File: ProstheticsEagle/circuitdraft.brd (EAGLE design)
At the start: 60 x 29.8 mm, 48 parts, among them IC1 BQ25887RGER, IC2 TPS54627DDAR, Q1 16 MHz

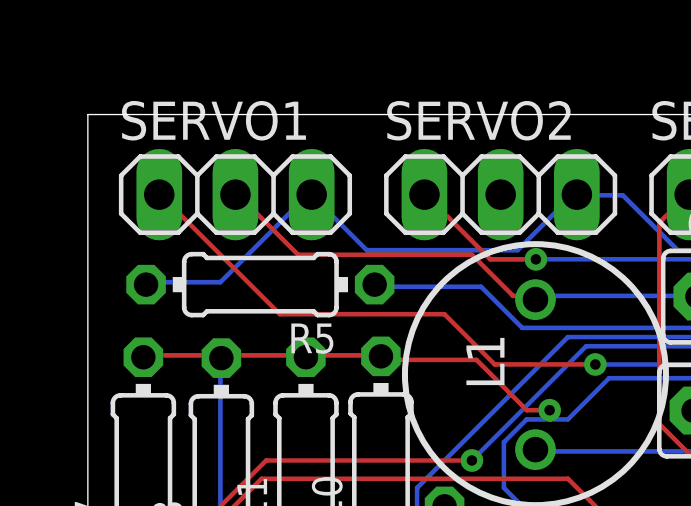
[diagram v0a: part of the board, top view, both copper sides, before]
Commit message: LED
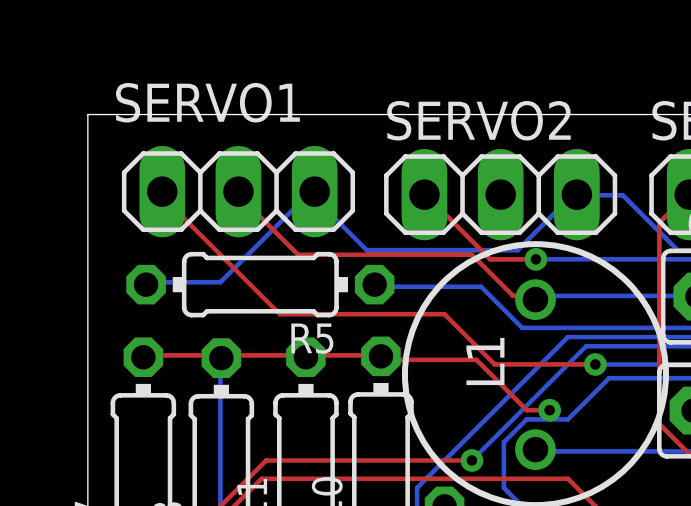
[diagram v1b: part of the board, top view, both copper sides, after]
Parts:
- moved SERVO1 0.14 mm to (5.02, 27.2)
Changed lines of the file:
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@@
 <drawing>
 <settings>
-<setting alwaysvectorfont="yes"/>
+<setting alwaysvectorfont="no"/>
 <setting verticaltext="up"/>
 </settings>
@@
 <attribute name="VALUE" x="35.0474" y="11.1456" size="0.9906" layer="27" ratio="10" rot="R270"/>
 </element>
-<element name="SERVO1" library="pinhead" library_urn="urn:adsk.eagle:library:325" package="1X03" package3d_urn="urn:adsk.eagle:package:22458/2" value="" x="4.92" y="27.15" smashed="yes">
-<attribute name="NAME" x="1.0338" y="28.9788" size="1.27" layer="25" ratio="10"/>
-<attribute name="POPULARITY" value="92" x="58.26" y="-18.57" size="1.778" layer="27" display="off"/>
-<attribute name="VALUE" x="1.11" y="23.975" size="1.27" layer="27"/>
+<element name="SERVO1" library="pinhead" library_urn="urn:adsk.eagle:library:325" package="1X03" package3d_urn="urn:adsk.eagle:package:22458/2" value="" x="5.02" y="27.25" smashed="yes">
+<attribute name="NAME" x="0.8338" y="29.5788" size="1.27" layer="25" ratio="10"/>
+<attribute name="POPULARITY" value="92" x="58.36" y="-18.47" size="1.778" layer="27" display="off"/>
+<attribute name="VALUE" x="1.21" y="24.075" size="1.27" layer="27"/>
 </element>
 <element name="SERVO2" library="pinhead" library_urn="urn:adsk.eagle:library:325" package="1X03" package3d_urn="urn:adsk.eagle:package:22458/2" value="" x="13.76" y="27.15" smashed="yes">
@@
 <wire x1="14.9352" y1="23.7744" x2="14.92" y2="23.65" width="0.1524" layer="16"/>
 <wire x1="20.2692" y1="23.7744" x2="20.32" y2="23.75" width="0.1524" layer="16"/>
-<wire x1="7.0104" y1="25.146" x2="5.0292" y2="27.1272" width="0.1524" layer="1"/>
+<wire x1="7.0104" y1="25.146" x2="5.049978125" y2="27.106421875" width="0.1524" layer="1"/>
 <wire x1="12.8016" y1="25.146" x2="7.0104" y2="25.146" width="0.1524" layer="1"/>
 <wire x1="14.1732" y1="23.7744" x2="12.8016" y2="25.146" width="0.1524" layer="1"/>
 <wire x1="14.7828" y1="23.7744" x2="14.1732" y2="23.7744" width="0.1524" layer="1"/>
-<wire x1="5.0292" y1="27.1272" x2="4.92" y2="27.15" width="0.1524" layer="1"/>
+<wire x1="5.049978125" y1="27.106421875" x2="5.02" y2="27.25" width="0.1524" layer="1"/>
 <wire x1="14.7828" y1="23.7744" x2="14.92" y2="23.65" width="0.1524" layer="1"/>
 <wire x1="22.5552" y1="25.908" x2="22.5552" y2="27.1272" width="0.1524" layer="1"/>
@@
 <wire x1="23.622" y1="10.8204" x2="23.56" y2="10.95" width="0.1524" layer="1"/>
 <wire x1="4.4196" y1="24.2316" x2="1.9812" y2="24.2316" width="0.1524" layer="16"/>
-<wire x1="7.3152" y1="27.1272" x2="4.4196" y2="24.2316" width="0.1524" layer="16"/>
+<wire x1="7.4152" y1="27.2272" x2="4.4196" y2="24.2316" width="0.1524" layer="16"/>
 <wire x1="1.9812" y1="24.2316" x2="1.94" y2="24.15" width="0.1524" layer="16"/>
-<wire x1="7.3152" y1="27.1272" x2="7.46" y2="27.15" width="0.1524" layer="16"/>
+<wire x1="7.4152" y1="27.2272" x2="7.56" y2="27.25" width="0.1524" layer="16"/>
 <wire x1="14.3256" y1="25.2984" x2="16.1544" y2="27.1272" width="0.1524" layer="16"/>
 <wire x1="9.2964" y1="25.2984" x2="14.3256" y2="25.2984" width="0.1524" layer="16"/>
-<wire x1="7.4676" y1="27.1272" x2="9.2964" y2="25.2984" width="0.1524" layer="16"/>
+<wire x1="7.6676" y1="26.9272" x2="9.2964" y2="25.2984" width="0.1524" layer="16"/>
 <wire x1="16.1544" y1="27.1272" x2="16.3" y2="27.15" width="0.1524" layer="16"/>
-<wire x1="7.4676" y1="27.1272" x2="7.46" y2="27.15" width="0.1524" layer="16"/>
+<wire x1="7.6676" y1="26.9272" x2="7.56" y2="27.25" width="0.1524" layer="16"/>
 <wire x1="25.146" y1="24.9936" x2="25.146" y2="27.1272" width="0.1524" layer="1"/>
 <wire x1="27.7368" y1="22.4028" x2="25.146" y2="24.9936" width="0.1524" layer="1"/>
@@
 <wire x1="11.8872" y1="23.1648" x2="13.5636" y2="21.4884" width="0.1524" layer="1"/>
 <wire x1="6.4008" y1="23.1648" x2="11.8872" y2="23.1648" width="0.1524" layer="1"/>
-<wire x1="2.4384" y1="27.1272" x2="6.4008" y2="23.1648" width="0.1524" layer="1"/>
+<wire x1="2.585290625" y1="26.980309375" x2="6.4008" y2="23.1648" width="0.1524" layer="1"/>
 <wire x1="51.6636" y1="22.86" x2="51.69" y2="22.79" width="0.1524" layer="1"/>
-<wire x1="2.4384" y1="27.1272" x2="2.38" y2="27.15" width="0.1524" layer="1"/>
+<wire x1="2.585290625" y1="26.980309375" x2="2.48" y2="27.25" width="0.1524" layer="1"/>
 <via x="46.9392" y="22.86" extent="1-16" drill="0.35"/>
 <via x="16.9164" y="21.4884" extent="1-16" drill="0.35"/>

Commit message: reste
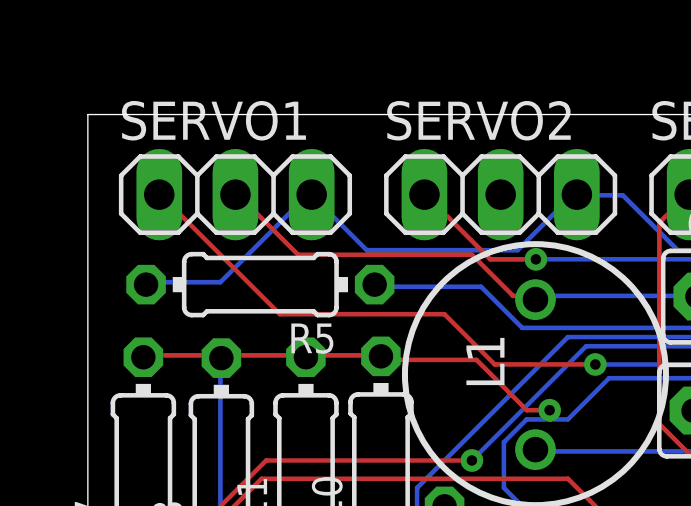
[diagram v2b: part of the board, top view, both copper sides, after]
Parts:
- moved SERVO1 0.14 mm to (4.92, 27.1)
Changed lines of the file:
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@@
 <drawing>
 <settings>
-<setting alwaysvectorfont="no"/>
+<setting alwaysvectorfont="yes"/>
 <setting verticaltext="up"/>
 </settings>
@@
 <attribute name="VALUE" x="35.0474" y="11.1456" size="0.9906" layer="27" ratio="10" rot="R270"/>
 </element>
-<element name="SERVO1" library="pinhead" library_urn="urn:adsk.eagle:library:325" package="1X03" package3d_urn="urn:adsk.eagle:package:22458/2" value="" x="5.02" y="27.25" smashed="yes">
-<attribute name="NAME" x="0.8338" y="29.5788" size="1.27" layer="25" ratio="10"/>
-<attribute name="POPULARITY" value="92" x="58.36" y="-18.47" size="1.778" layer="27" display="off"/>
-<attribute name="VALUE" x="1.21" y="24.075" size="1.27" layer="27"/>
+<element name="SERVO1" library="pinhead" library_urn="urn:adsk.eagle:library:325" package="1X03" package3d_urn="urn:adsk.eagle:package:22458/2" value="" x="4.92" y="27.15" smashed="yes">
+<attribute name="NAME" x="1.0338" y="28.9788" size="1.27" layer="25" ratio="10"/>
+<attribute name="POPULARITY" value="92" x="58.26" y="-18.57" size="1.778" layer="27" display="off"/>
+<attribute name="VALUE" x="1.11" y="23.975" size="1.27" layer="27"/>
 </element>
 <element name="SERVO2" library="pinhead" library_urn="urn:adsk.eagle:library:325" package="1X03" package3d_urn="urn:adsk.eagle:package:22458/2" value="" x="13.76" y="27.15" smashed="yes">
@@
 <wire x1="14.9352" y1="23.7744" x2="14.92" y2="23.65" width="0.1524" layer="16"/>
 <wire x1="20.2692" y1="23.7744" x2="20.32" y2="23.75" width="0.1524" layer="16"/>
-<wire x1="7.0104" y1="25.146" x2="5.049978125" y2="27.106421875" width="0.1524" layer="1"/>
+<wire x1="7.0104" y1="25.146" x2="5.0292" y2="27.1272" width="0.1524" layer="1"/>
 <wire x1="12.8016" y1="25.146" x2="7.0104" y2="25.146" width="0.1524" layer="1"/>
 <wire x1="14.1732" y1="23.7744" x2="12.8016" y2="25.146" width="0.1524" layer="1"/>
 <wire x1="14.7828" y1="23.7744" x2="14.1732" y2="23.7744" width="0.1524" layer="1"/>
-<wire x1="5.049978125" y1="27.106421875" x2="5.02" y2="27.25" width="0.1524" layer="1"/>
+<wire x1="5.0292" y1="27.1272" x2="4.92" y2="27.15" width="0.1524" layer="1"/>
 <wire x1="14.7828" y1="23.7744" x2="14.92" y2="23.65" width="0.1524" layer="1"/>
 <wire x1="22.5552" y1="25.908" x2="22.5552" y2="27.1272" width="0.1524" layer="1"/>
@@
 <wire x1="23.622" y1="10.8204" x2="23.56" y2="10.95" width="0.1524" layer="1"/>
 <wire x1="4.4196" y1="24.2316" x2="1.9812" y2="24.2316" width="0.1524" layer="16"/>
-<wire x1="7.4152" y1="27.2272" x2="4.4196" y2="24.2316" width="0.1524" layer="16"/>
+<wire x1="7.3152" y1="27.1272" x2="4.4196" y2="24.2316" width="0.1524" layer="16"/>
 <wire x1="1.9812" y1="24.2316" x2="1.94" y2="24.15" width="0.1524" layer="16"/>
-<wire x1="7.4152" y1="27.2272" x2="7.56" y2="27.25" width="0.1524" layer="16"/>
+<wire x1="7.3152" y1="27.1272" x2="7.46" y2="27.15" width="0.1524" layer="16"/>
 <wire x1="14.3256" y1="25.2984" x2="16.1544" y2="27.1272" width="0.1524" layer="16"/>
 <wire x1="9.2964" y1="25.2984" x2="14.3256" y2="25.2984" width="0.1524" layer="16"/>
-<wire x1="7.6676" y1="26.9272" x2="9.2964" y2="25.2984" width="0.1524" layer="16"/>
+<wire x1="7.4676" y1="27.1272" x2="9.2964" y2="25.2984" width="0.1524" layer="16"/>
 <wire x1="16.1544" y1="27.1272" x2="16.3" y2="27.15" width="0.1524" layer="16"/>
-<wire x1="7.6676" y1="26.9272" x2="7.56" y2="27.25" width="0.1524" layer="16"/>
+<wire x1="7.4676" y1="27.1272" x2="7.46" y2="27.15" width="0.1524" layer="16"/>
 <wire x1="25.146" y1="24.9936" x2="25.146" y2="27.1272" width="0.1524" layer="1"/>
 <wire x1="27.7368" y1="22.4028" x2="25.146" y2="24.9936" width="0.1524" layer="1"/>
@@
 <wire x1="11.8872" y1="23.1648" x2="13.5636" y2="21.4884" width="0.1524" layer="1"/>
 <wire x1="6.4008" y1="23.1648" x2="11.8872" y2="23.1648" width="0.1524" layer="1"/>
-<wire x1="2.585290625" y1="26.980309375" x2="6.4008" y2="23.1648" width="0.1524" layer="1"/>
+<wire x1="2.4384" y1="27.1272" x2="6.4008" y2="23.1648" width="0.1524" layer="1"/>
 <wire x1="51.6636" y1="22.86" x2="51.69" y2="22.79" width="0.1524" layer="1"/>
-<wire x1="2.585290625" y1="26.980309375" x2="2.48" y2="27.25" width="0.1524" layer="1"/>
+<wire x1="2.4384" y1="27.1272" x2="2.38" y2="27.15" width="0.1524" layer="1"/>
 <via x="46.9392" y="22.86" extent="1-16" drill="0.35"/>
 <via x="16.9164" y="21.4884" extent="1-16" drill="0.35"/>
